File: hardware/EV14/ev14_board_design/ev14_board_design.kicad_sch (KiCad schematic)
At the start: 173 parts, among them CN1 Conn_05x02_Female, J1 USB_C_Receptacle, J10 Conn_02x05_Counter_Clockwise, J2 Conn_01x02_Socket, J3 AudioJack4, J4 AudioJack4, J5 Conn_02x03_Odd_Even, J6 Conn_01x35_Socket, J7 Conn_02x05_Counter_Clockwise, J8 Conn_02x05_Counter_Clockwise, J9 Conn_02x05_Counter_Clockwise, Q1 2N7002, Q2 Q_Dual_NMOS_S1G1D2S2G2D1, Q3 PMOS, SW1 SW_SPDT, SW2 SW_Push, SW3 SW_Push, SW4 SW_Push, SW5 SW_Push, U1 BQ21040DBV, U10 STM32F405RGTx, U2 USBLC6-2P6, U3 STM32F072CBTx, U4 CH340C, U5 TPS63060, U6 WM8960CGEFL/RV, U7 ESP32-S3-WROOM-1, U8 M24C02-RMN6TP, U9 BM14B(0.8)-24DS-0.4V(53), Y1 Crystal_GND24

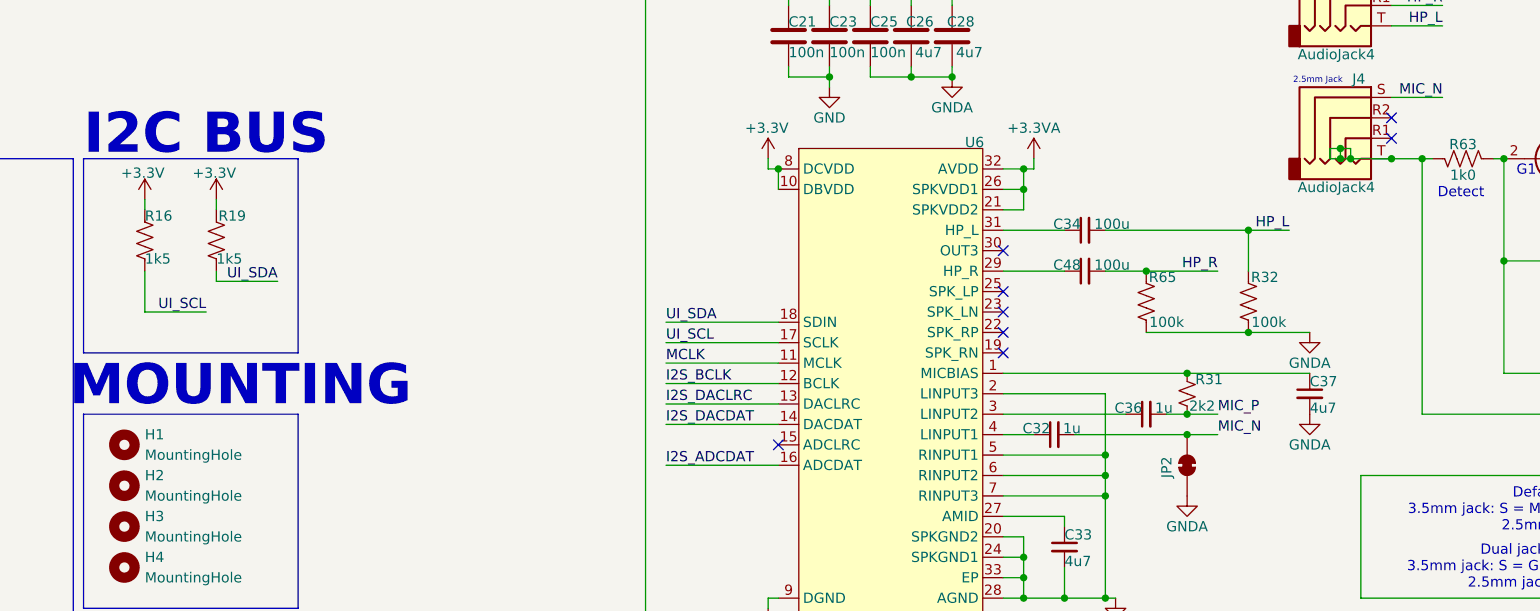
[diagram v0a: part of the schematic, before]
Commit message: Latest version of Ev14
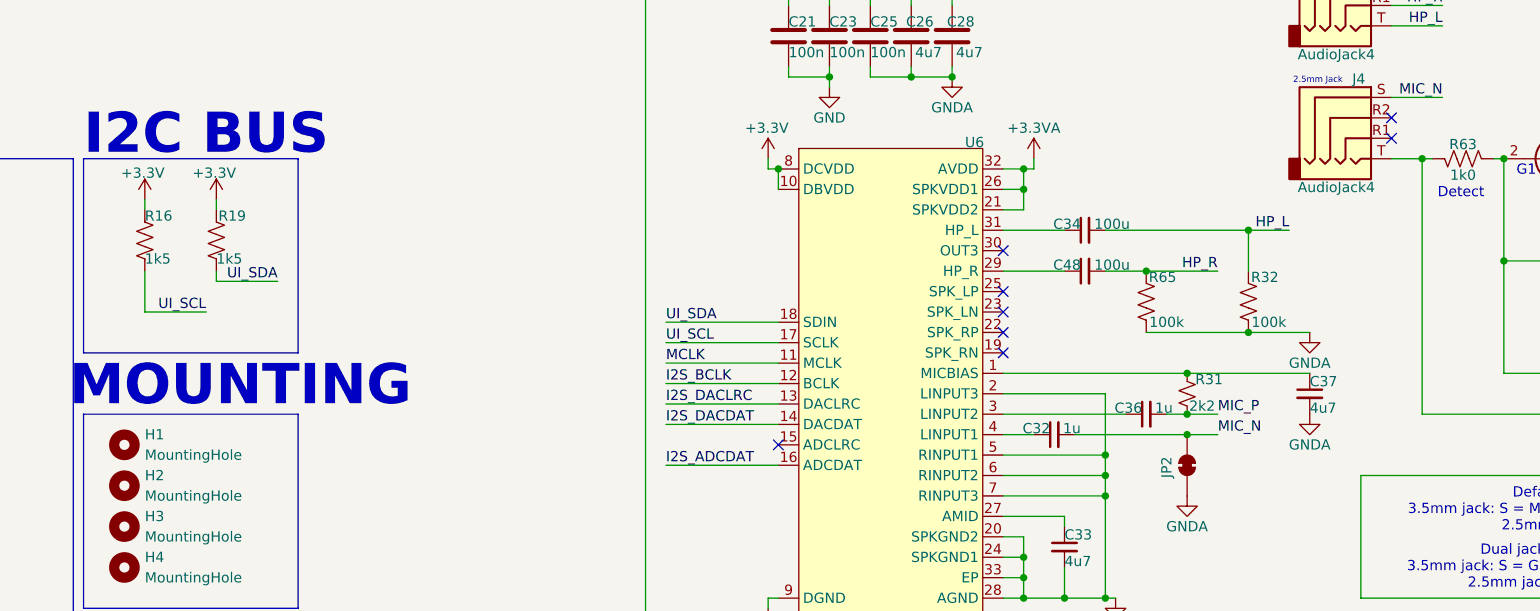
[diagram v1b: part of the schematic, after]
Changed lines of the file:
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@@
 	)
 	(junction
-		(at 299.72 191.77)
-		(diameter 0)
-		(color 0 0 0 0)
-	)
-	(junction
 		(at 265.43 351.79)
 		(diameter 0)
@@
 	)
 	(junction
-		(at 298.45 191.77)
-		(diameter 0)
-		(color 0 0 0 0)
-	)
-	(junction
 		(at 40.64 68.58)
 		(diameter 0)
@@
 	)
 	(junction
-		(at 304.8 191.77)
-		(diameter 0)
-		(color 0 0 0 0)
-	)
-	(junction
 		(at 57.15 240.03)
 		(diameter 0)
@@
 	)
 	(junction
-		(at 298.45 190.5)
-		(diameter 0)
-		(color 0 0 0 0)
-	)
-	(junction
 		(at 240.03 170.18)
 		(diameter 0)
@@
 	(wire
 		(pts
-			(xy 304.8 191.77) (xy 299.72 191.77)
-		)
-		(stroke
-			(width 0)
-			(type default)
-		)
-	)
-	(wire
-		(pts
 			(xy 464.82 214.63) (xy 464.82 213.36)
 		)
@@
 	(wire
 		(pts
-			(xy 298.45 191.77) (xy 297.18 191.77)
-		)
-		(stroke
-			(width 0)
-			(type default)
-		)
-	)
-	(wire
-		(pts
 			(xy 250.19 181.61) (xy 245.11 181.61)
 		)
@@
 	(wire
 		(pts
-			(xy 299.72 191.77) (xy 299.72 190.5)
-		)
-		(stroke
-			(width 0)
-			(type default)
-		)
-	)
-	(wire
-		(pts
 			(xy 265.43 226.06) (xy 279.4 226.06)
 		)
@@
 	(wire
 		(pts
-			(xy 299.72 191.77) (xy 298.45 191.77)
-		)
-		(stroke
-			(width 0)
-			(type default)
-		)
-	)
-	(wire
-		(pts
 			(xy 214.63 229.87) (xy 228.6 229.87)
 		)
@@
 	(wire
 		(pts
-			(xy 298.45 191.77) (xy 298.45 190.5)
-		)
-		(stroke
-			(width 0)
-			(type default)
-		)
-	)
-	(wire
-		(pts
 			(xy 553.72 91.44) (xy 558.8 91.44)
 		)
@@
 	(wire
 		(pts
-			(xy 299.72 190.5) (xy 298.45 190.5)
-		)
-		(stroke
-			(width 0)
-			(type default)
-		)
-	)
-	(wire
-		(pts
 			(xy 219.71 322.58) (xy 227.33 322.58)
 		)
@@
 		)
 	)
-	(wire
-		(pts
-			(xy 297.18 190.5) (xy 298.45 190.5)
-		)
-		(stroke
-			(width 0)
-			(type default)
-		)
-	)
 	(polyline
 		(pts
@@
 	(wire
 		(pts
-			(xy 297.18 191.77) (xy 297.18 190.5)
-		)
-		(stroke
-			(width 0)
-			(type default)
-		)
-	)
-	(wire
-		(pts
 			(xy 213.36 336.55) (xy 213.36 340.36)
 		)
@@
 		(on_board yes)
 		(dnp no)
-		(fields_autoplaced yes)
 		(property "Reference" "H1"
 			(at 149.86 226.0599 0)
@@
 		)
 		(property "Value" "MountingHole"
-			(at 149.86 228.5999 0)
+			(at 149.86 228.6 0)
 			(effects
 				(font
